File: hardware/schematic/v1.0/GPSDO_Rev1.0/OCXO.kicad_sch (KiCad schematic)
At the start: 24 parts, among them U2 LMK1C1103PWR, U3 TMP117AIDRVR, U5 OCXO_20x20mm, U7 OCXO_25.4x25.4mm, U8 REF5040

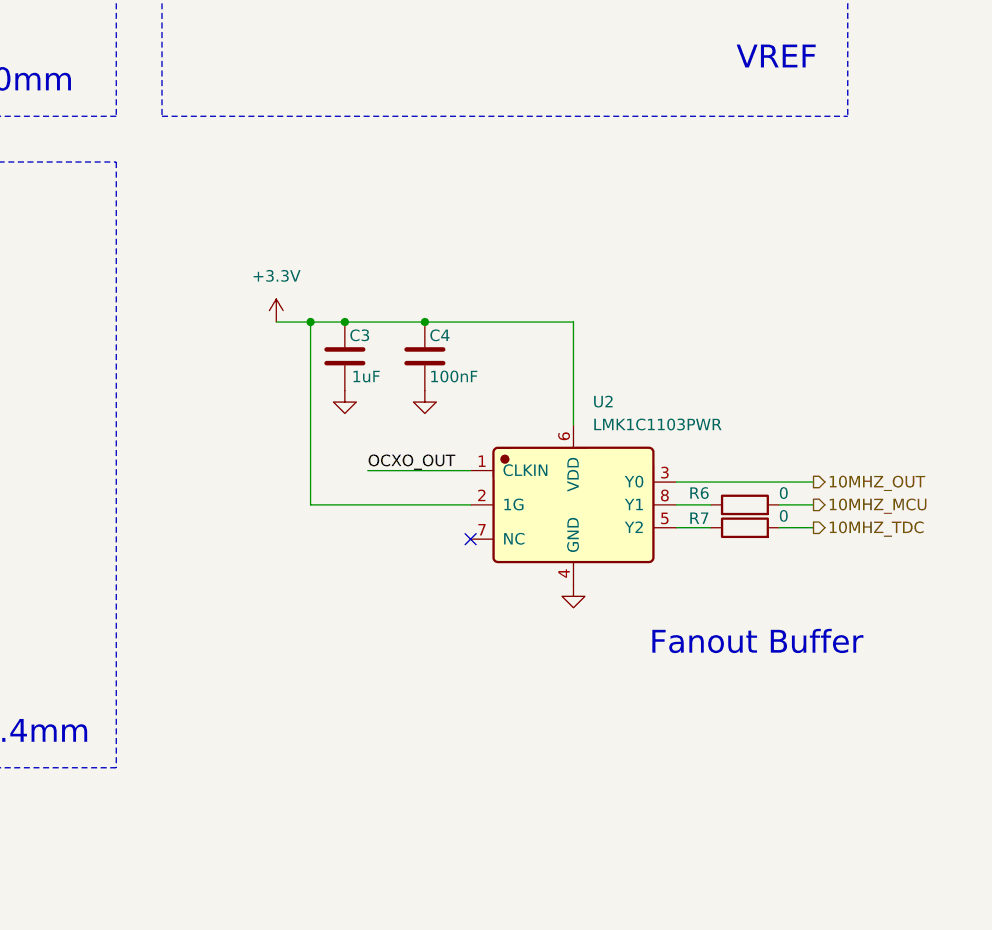
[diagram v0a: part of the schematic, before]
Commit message: sch update
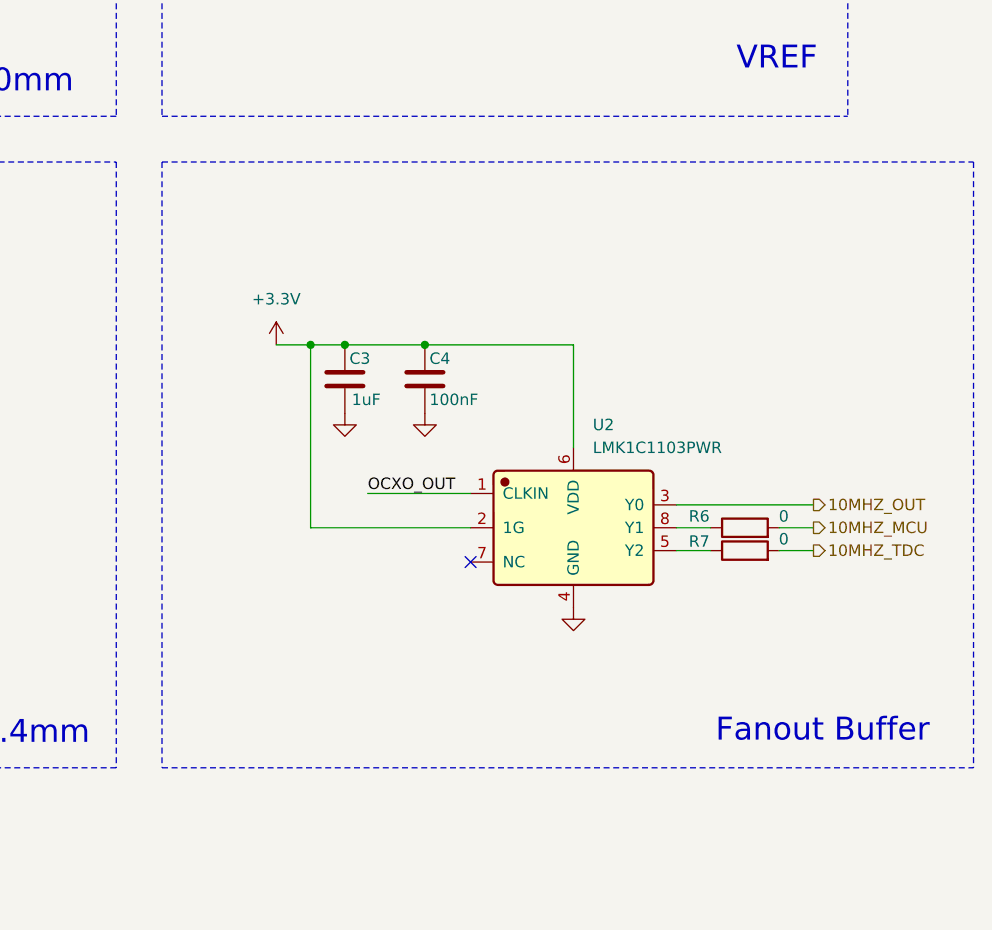
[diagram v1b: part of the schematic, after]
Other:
- moved on the sheet: C3, C4, R6, R7, U2

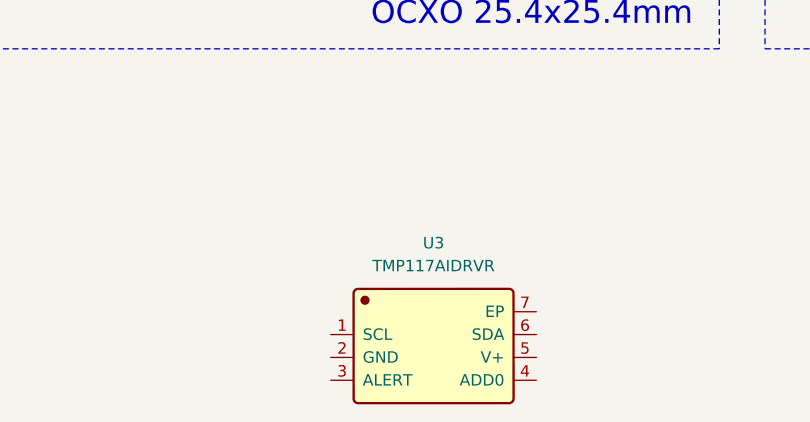
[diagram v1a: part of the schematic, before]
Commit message: pdf and sch update
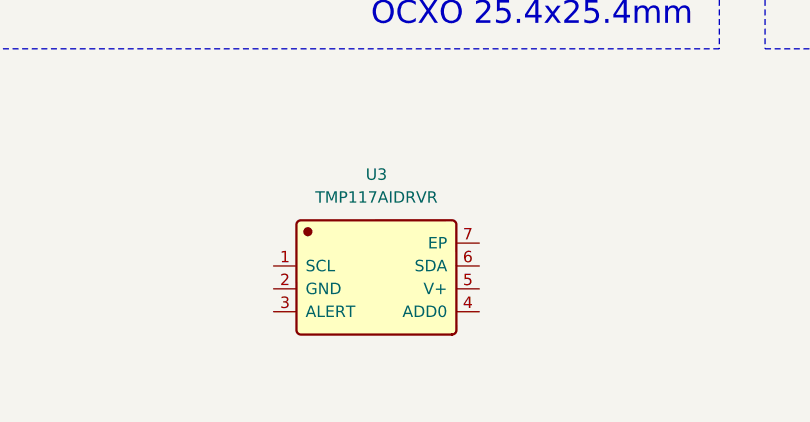
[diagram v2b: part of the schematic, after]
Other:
- moved on the sheet: U3
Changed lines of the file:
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@@
 	(symbol
 		(lib_id "GPSDO_Rev1.0:TMP117AIDRVR")
-		(at 148.59 181.61 0)
+		(at 142.24 173.99 0)
 		(unit 1)
 		(body_style 1)
@@
 		(fields_autoplaced yes)
 		(property "Reference" "U3"
-			(at 148.59 170.18 0)
+			(at 142.24 162.56 0)
 			(show_name no)
 			(do_not_autoplace no)
@@
 		)
 		(property "Value" "TMP117AIDRVR"
-			(at 148.59 172.72 0)
+			(at 142.24 165.1 0)
 			(show_name no)
 			(do_not_autoplace no)
@@
 		)
 		(property "Footprint" "GPSDO_Rev1.0:TMP117AIDRVR"
-			(at 148.59 181.61 0)
+			(at 142.24 173.99 0)
 			(hide yes)
 			(show_name no)
@@
 		)
 		(property "Datasheet" "https://www.lcsc.com/datasheet/lcsc_datasheet_2309221403_Texas-Instruments-TMP117AIDRVR_C699536.pdf"
-			(at 148.59 181.61 0)
+			(at 142.24 173.99 0)
 			(hide yes)
 			(show_name no)
@@
 		)
 		(property "Description" "-55℃~+150℃ 1.7V~5.5V 15.5ms 16bit 3.1uA Factory temperature calibration、Temperature threshold monitoring、Low-power standby、On-chip non-volatile parameter storage、On-chip digital filtering/averaging I2C、SMBus ±0.1℃ WDFN-6-EP(2x2) Temperature Sensors ROHS"
-			(at 148.59 181.61 0)
+			(at 142.24 173.99 0)
 			(hide yes)
 			(show_name no)
@@
 		)
 		(property "LCSC" "C699536"
-			(at 148.59 181.61 0)
+			(at 142.24 173.99 0)
 			(hide yes)
 			(show_name no)
@@
 		)
 		(property "Manufacturer" "Texas Instruments"
-			(at 148.59 181.61 0)
+			(at 142.24 173.99 0)
 			(hide yes)
 			(show_name no)
@@
 		)
 		(property "Manufacturer Part" "TMP117AIDRVR"
-			(at 148.59 181.61 0)
+			(at 142.24 173.99 0)
 			(hide yes)
 			(show_name no)
